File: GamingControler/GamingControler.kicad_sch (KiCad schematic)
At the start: 38 parts, among them J1 USB_C_Receptacle_USB2.0_16P, J2 USB_C_Receptacle_USB2.0_16P, SW1 SW_Push, SW2 SW_Push, U1 ESP32-C6-WROOM-1, U2 AZ1117-3.3, U3 CP2102N-Axx-xQFN20, U4 BME680

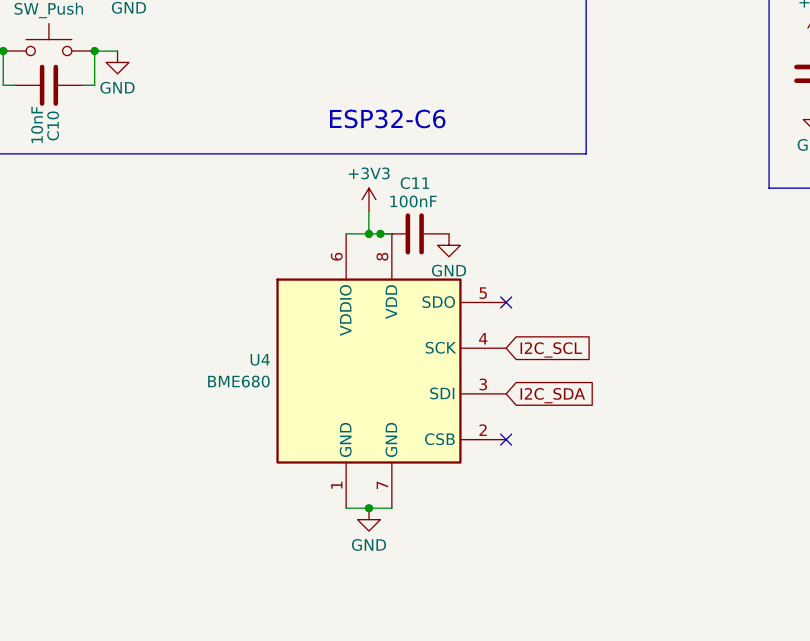
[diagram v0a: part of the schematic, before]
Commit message: GamingBoard
Created prototype of PCB
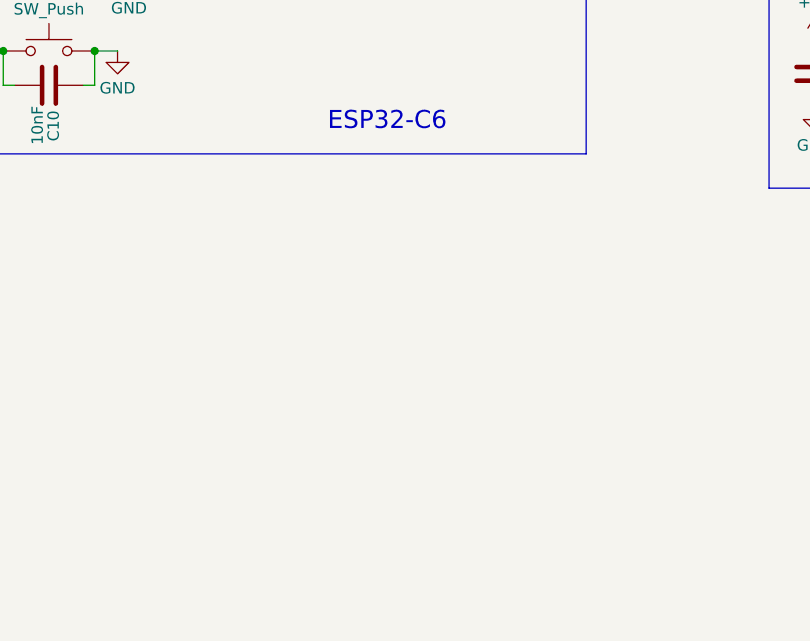
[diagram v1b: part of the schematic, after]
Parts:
- removed C11: 100nF, symbol Device:C
- removed U4: BME680, Package_LGA:Bosch_LGA-8_3x3mm_P0.8mm_ClockwisePinNumbering, symbol Sensor:BME680
- C1, C10, C2, C3, C4, C5, C6, C7, C8, C9: footprint (none) -> Capacitor_SMD:C_0805_2012Metric
- D1, D2, D3, D4, D5, D6: footprint Diode_THT:D_DO-201AE_P15.24mm_Horizontal -> Diode_SMD:D_SOD-523
- D7, D8: footprint (none) -> Diode_SMD:D_0805_2012Metric
- J1, J2: footprint (none) -> Connector_USB:USB_C_Receptacle_G-Switch_GT-USB-7010ASV
- JP1, JP2: footprint (none) -> Jumper:SolderJumper-2_P1.3mm_Open_TrianglePad1.0x1.5mm
- R1, R2, R3, R4, R5, R6, R7, R8, R9: footprint (none) -> Resistor_SMD:R_0805_2012Metric
- SW1, SW2: footprint (none) -> Button_Switch_SMD:SW_Push_1P1T_NO_6x6mm_H9.5mm
- U2: footprint (none) -> Package_TO_SOT_SMD:TO-252-2
- U3: footprint Package_DFN_QFN:SiliconLabs_QFN-20-1EP_3x3mm_P0.5mm -> Package_DFN_QFN:SiliconLabs_QFN-20-1EP_3x3mm_P0.5mm_EP1.8x1.8mm_ThermalVias
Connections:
- no-connect marks 14 -> 12

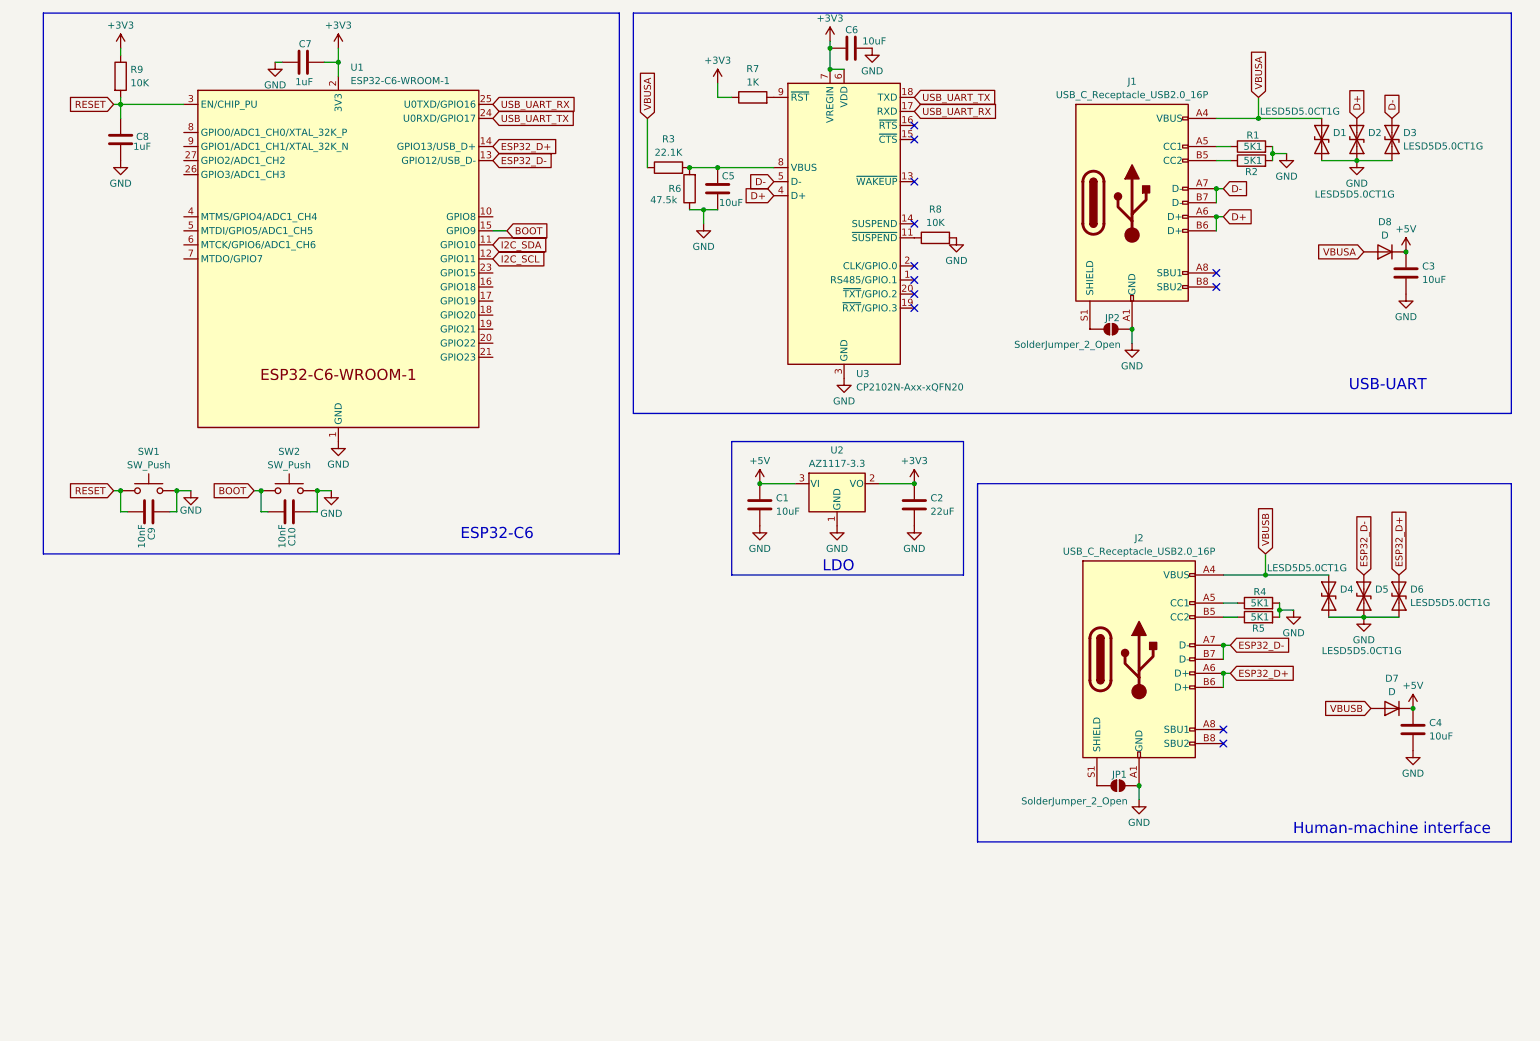
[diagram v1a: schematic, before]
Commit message: Final board
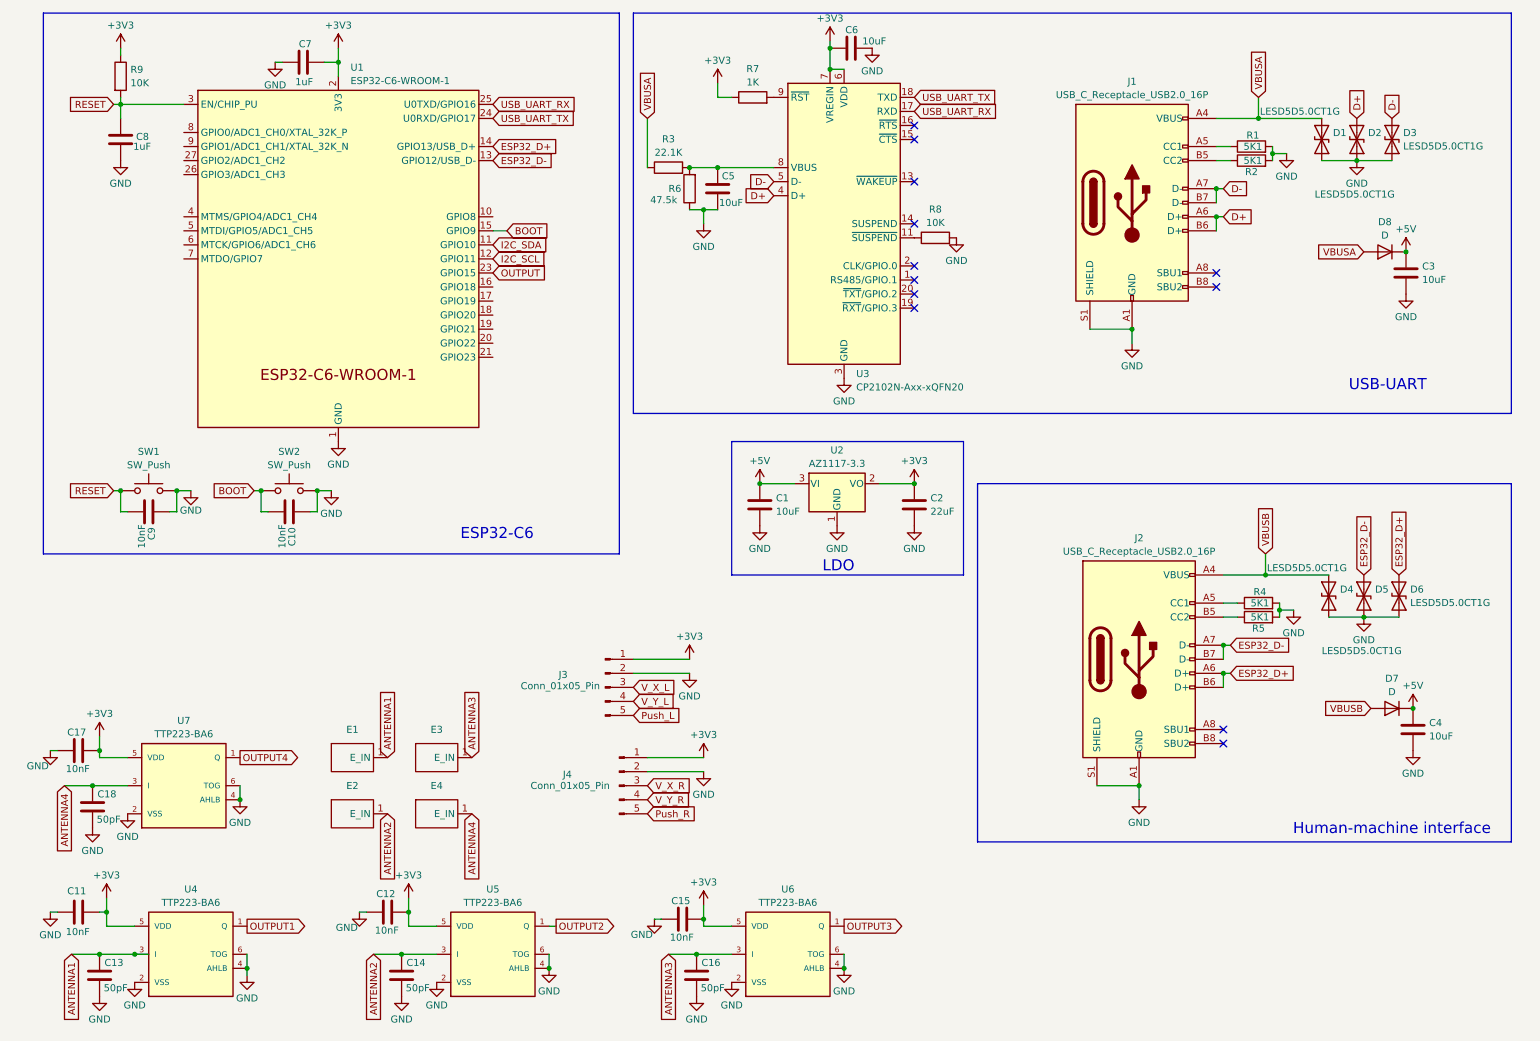
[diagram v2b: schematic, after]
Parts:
- removed JP1, JP2: SolderJumper_2_Open, Jumper:SolderJumper-2_P1.3mm_Open_TrianglePad1.0x1.5mm, symbol Jumper:SolderJumper_2_Open
- added C11, C12, C15, C17: 10nF, Capacitor_SMD:C_0805_2012Metric, symbol Device:C
- added C13, C14, C16, C18: 50pF, Capacitor_SMD:C_0805_2012Metric, symbol Device:C
- added E1, E2, E3, E4: ~, LED_SMD:Electrode_10x10mm, symbol Captive:Electrode
- added J3, J4: Conn_01x05_Pin, Connector_PinHeader_2.54mm:PinHeader_1x05_P2.54mm_Vertical, symbol Connector:Conn_01x05_Pin
- added U4, U5, U6, U7: TTP223-BA6, Package_TO_SOT_SMD:TSOT-23-6_HandSoldering, symbol TTP223-BA6:TTP223-BA6
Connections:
- net +3V3: now also C11.1, C12.1, C15.1, C17.1, J3.1 (Pin_1), J4.1 (Pin_1), U4.5 (VDD), U5.5 (VDD), U6.5 (VDD), U7.5 (VDD)
- net GND: now also J1.S1 (SHIELD), J2.S1 (SHIELD), C11.2, C12.2, C13.1, C14.1, C15.2, C16.1, C17.2, C18.1, J3.2 (Pin_2), J4.2 (Pin_2), U4.2 (VSS), U4.4 (AHLB), U4.6 (TOG), U5.2 (VSS), U5.4 (AHLB), U5.6 (TOG), U6.2 (VSS), U6.4 (AHLB), U6.6 (TOG), U7.2 (VSS), U7.4 (AHLB), U7.6 (TOG)
- net OUTPUT: now reaches U1.23 (GPIO15)
- new net ANTENNA1: C13.2, E1.1 (E_IN), U4.3 (I)
- new net ANTENNA2: C14.2, E2.1 (E_IN), U5.3 (I)
- new net ANTENNA3: C16.2, E3.1 (E_IN), U6.3 (I)
- new net ANTENNA4: C18.2, E4.1 (E_IN), U7.3 (I)
- new net OUTPUT1: U4.1 (Q)
- new net OUTPUT2: U5.1 (Q)
- new net OUTPUT3: U6.1 (Q)
- new net OUTPUT4: U7.1 (Q)
- new net Push_L: J3.5 (Pin_5)
- new net Push_R: J4.5 (Pin_5)
- new net V_X_L: J3.3 (Pin_3)
- new net V_X_R: J4.3 (Pin_3)
- new net V_Y_L: J3.4 (Pin_4)
- new net V_Y_R: J4.4 (Pin_4)

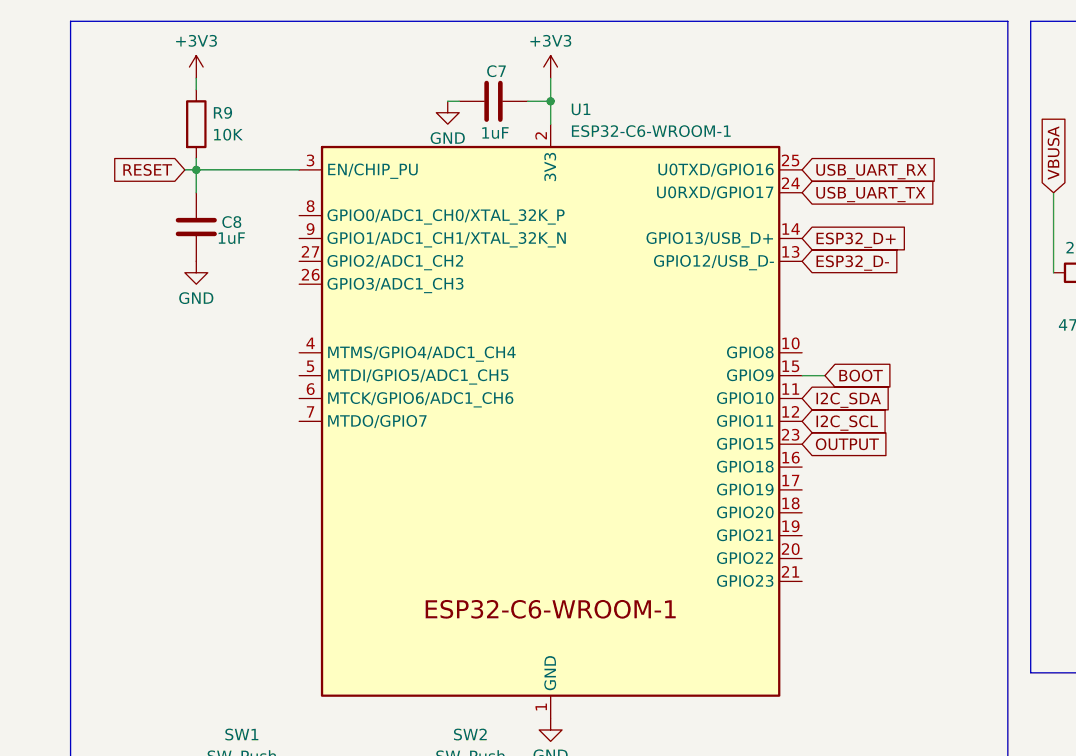
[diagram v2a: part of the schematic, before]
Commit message: summary
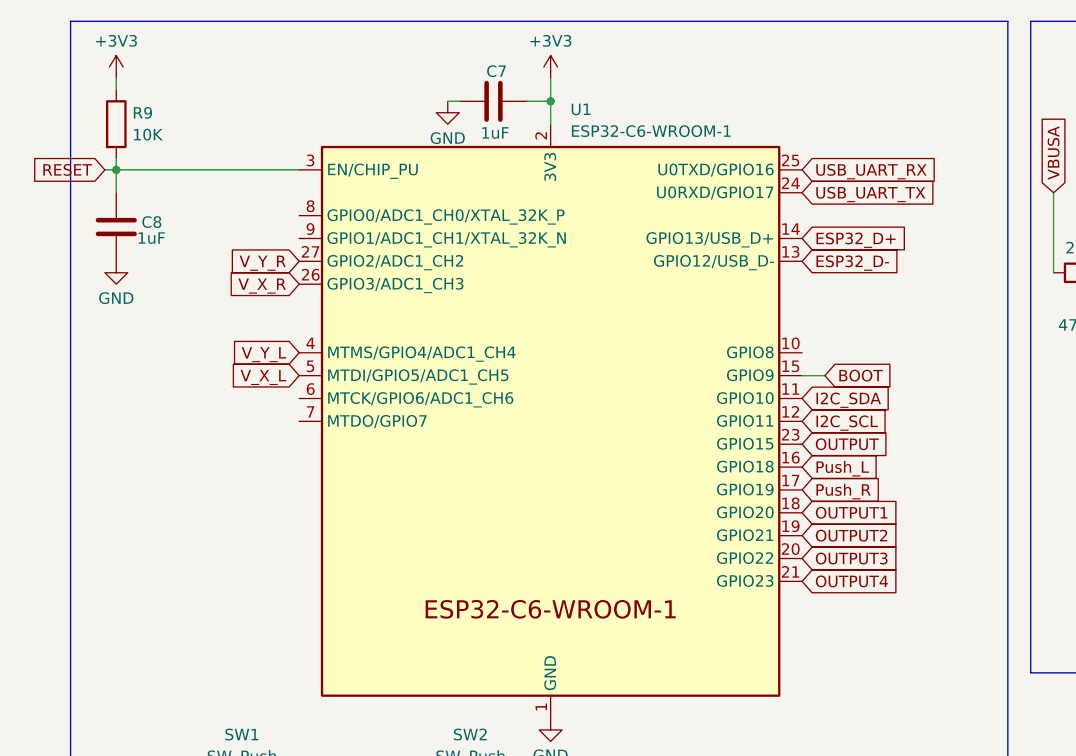
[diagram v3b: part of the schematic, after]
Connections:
- net OUTPUT1: now also U1.18 (GPIO20)
- net OUTPUT2: now also U1.19 (GPIO21)
- net OUTPUT3: now also U1.20 (GPIO22)
- net OUTPUT4: now also U1.21 (GPIO23)
- net Push_L: now also U1.16 (GPIO18)
- net Push_R: now also U1.17 (GPIO19)
- net V_X_L: now also U1.5 (MTDI/GPIO5/ADC1_CH5)
- net V_X_R: now also U1.26 (GPIO3/ADC1_CH3)
- net V_Y_L: now also U1.4 (MTMS/GPIO4/ADC1_CH4)
- net V_Y_R: now also U1.27 (GPIO2/ADC1_CH2)
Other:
- moved on the sheet: C8, R9
